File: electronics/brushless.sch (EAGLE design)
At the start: 70 parts, among them J1 USB_MINI-B_SMT, Q1 BUK7Y12-40E, Q2 BUK7Y12-40E, Q3 BUK7Y12-40E, Q4 BUK7Y12-40E, Q5 BUK7Y12-40E, Q6 BUK7Y12-40E, X1 JST-XH-10-PIN-LONG-PAD

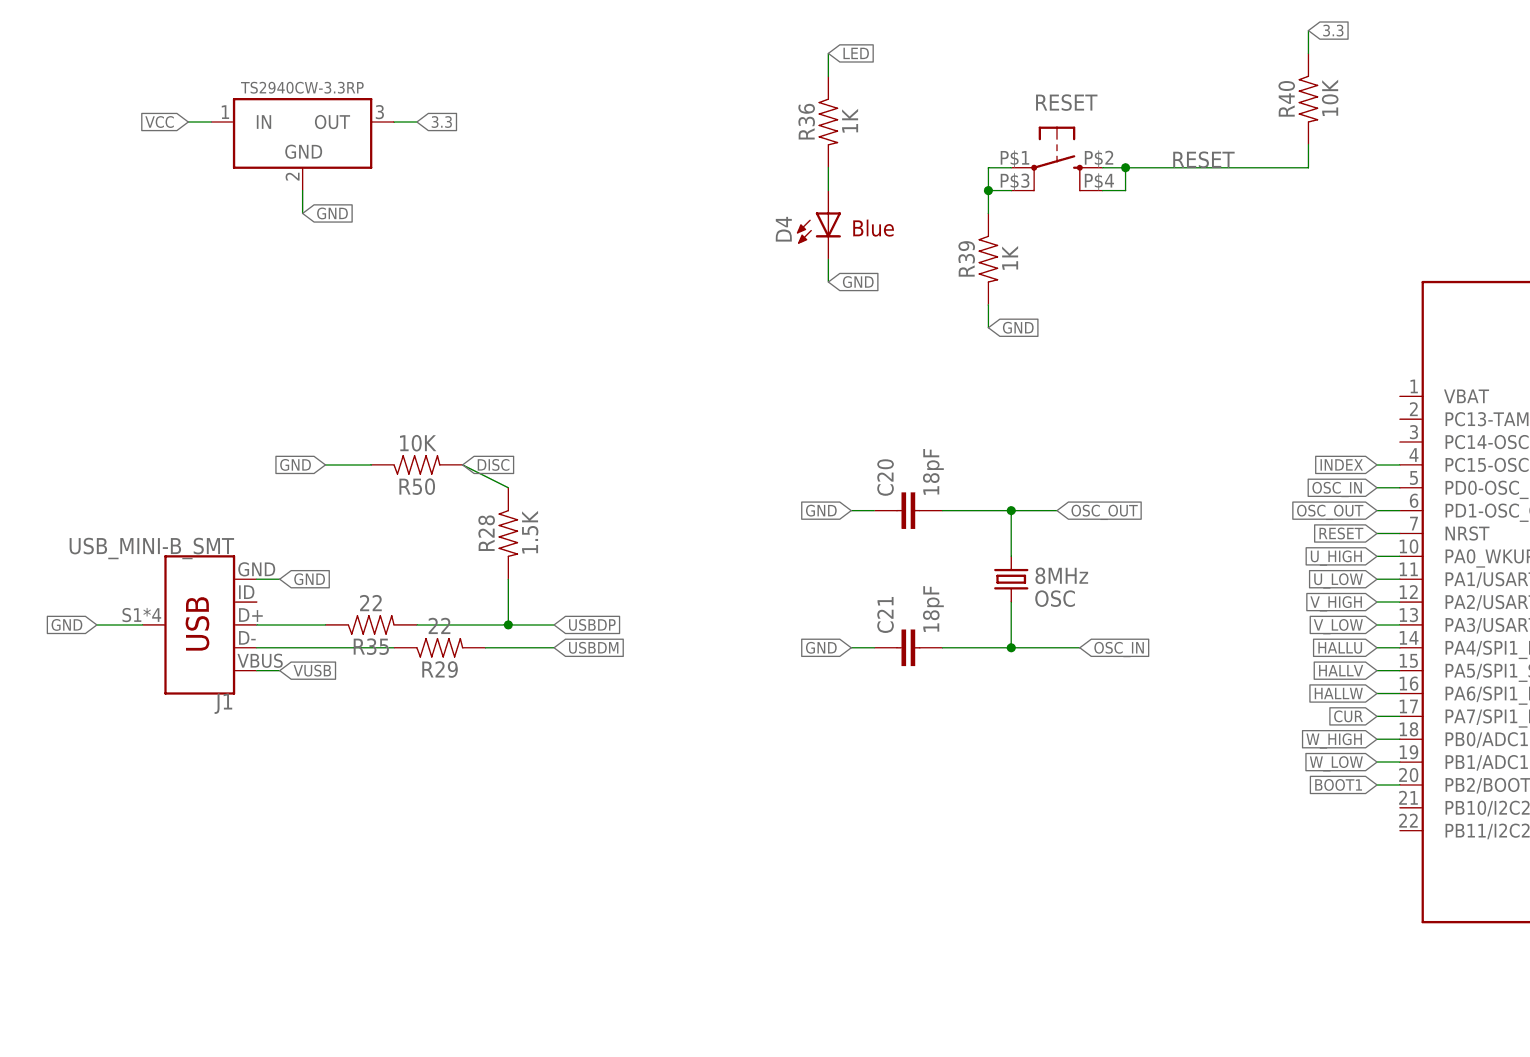
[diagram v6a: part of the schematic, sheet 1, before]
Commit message: Farnell refs & names
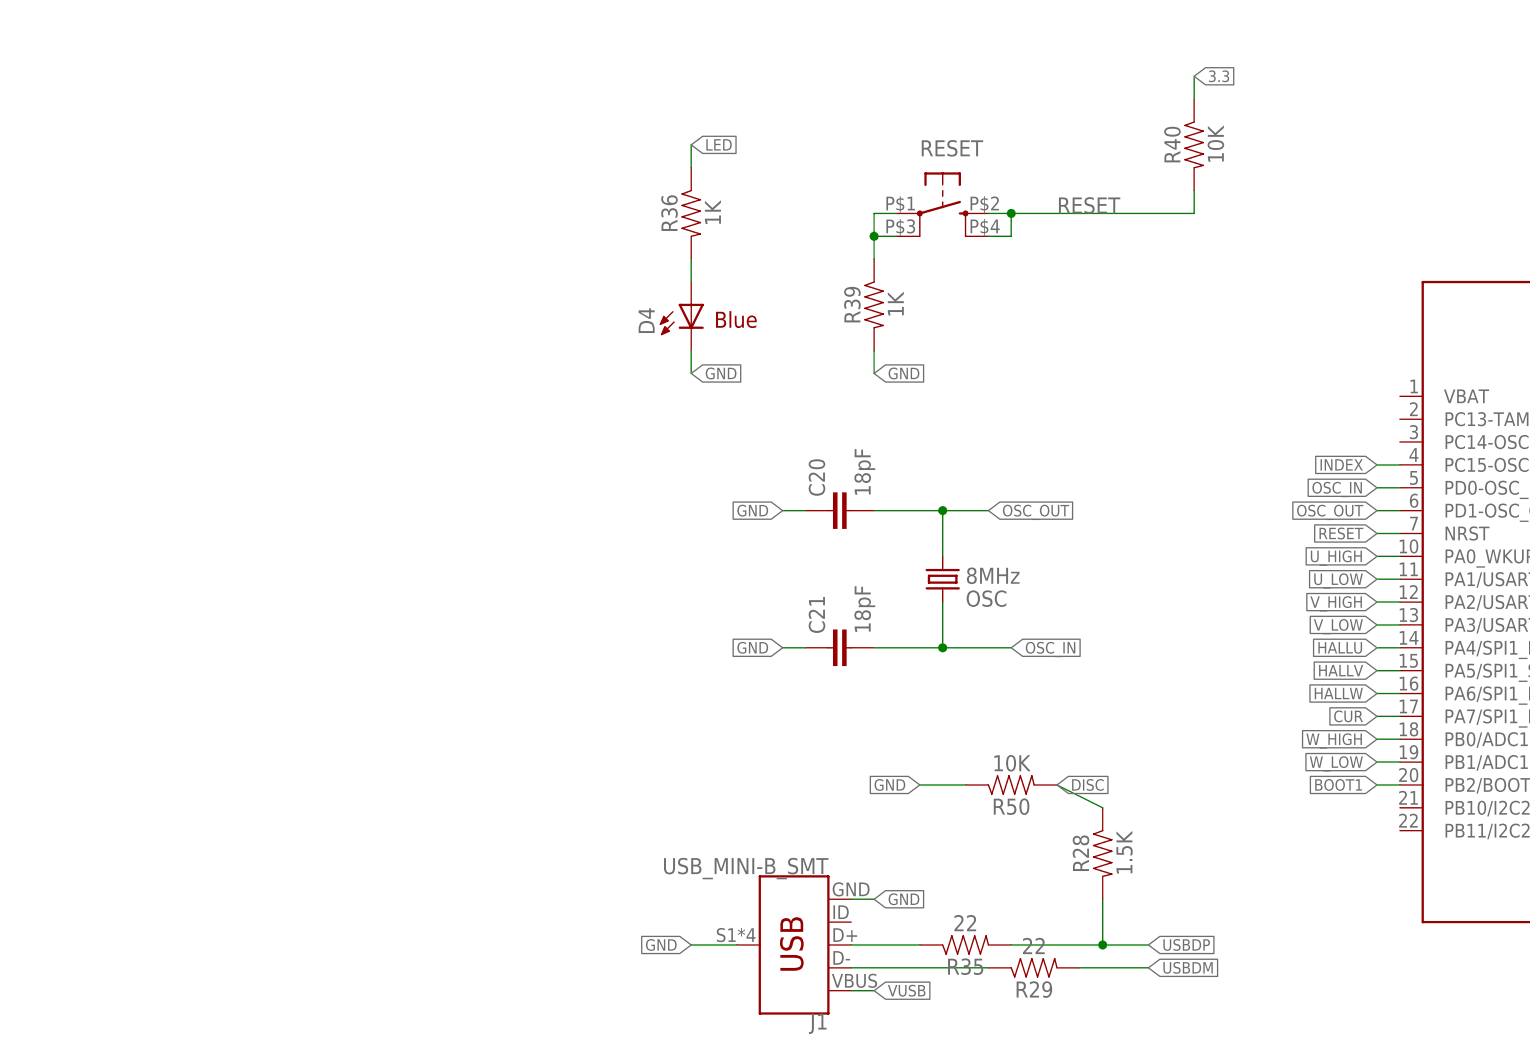
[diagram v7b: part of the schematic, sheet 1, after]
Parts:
- removed U$4: TS2940CW-3.3RP, rhoban:TS2940CW-3.3RP
- added REG1: TS2940CW-3.3RP, rhoban:TS2940CW-3.3RP
- BUT, RESET: FARNELL (none) -> 1437637
- C1, C2, C3: FARNELL (none) -> 2528772
- C12, C7: FARNELL (none) -> 2496946
- C17, C18: FARNELL (none) -> 721980
- C20, C21: FARNELL (none) -> 1414620
- C4: value 1nF -> 1000pF; FARNELL (none) -> 2496935
- D4: FARNELL (none) -> 1581233
- ENC1, R13, X1: FARNELL (none) -> -
- GND, V+: FARNELL (none) -> 1022248
- J1: FARNELL (none) -> 1753807
- LOGIC: FARNELL (none) -> 1022256
- OSC: FARNELL (none) -> 2467818
- OSC1: FARNELL (none) -> 1842013
- Q1, Q2, Q3, Q4, Q5, Q6: FARNELL (none) -> 2319916
- R1, R2, R3, R36, R39, R4, R49, R5, R6: FARNELL (none) -> 2446904
- R10, R11, R12, R14, R15, R16, R17, R18, R19, R23, R24, R25, R40, R48, R50, R7, R8, R9: FARNELL (none) -> 2447553
- R20: FARNELL (none) -> 2446939
- R21: FARNELL (none) -> 2446965
- R28: FARNELL (none) -> 2446909
- R29, R35: FARNELL (none) -> 2446926
- U$6: value (none) -> 100uF; FARNELL (none) -> 1144713
- U$7: FARNELL (none) -> 1329624
- renumbered U$1 to DRV1, U$2 to DRV2, U$3 to DRV3, U$5 to LOGIC
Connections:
- net 3.3: now also REG1.OUT; no longer U$4.OUT
- net GND: now also REG1.GND; no longer U$4.GND
- net VCC: now also REG1.IN; no longer U$4.IN
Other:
- note added: "CONNECTORS & POWER"
- note added: "STM32"
- note removed: "CONNECTORS"
- note removed: "MCU"
- moved on the sheet: C20, C21, D4, J1, OSC, R23, R24, R25, R28, R29, R35, R36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

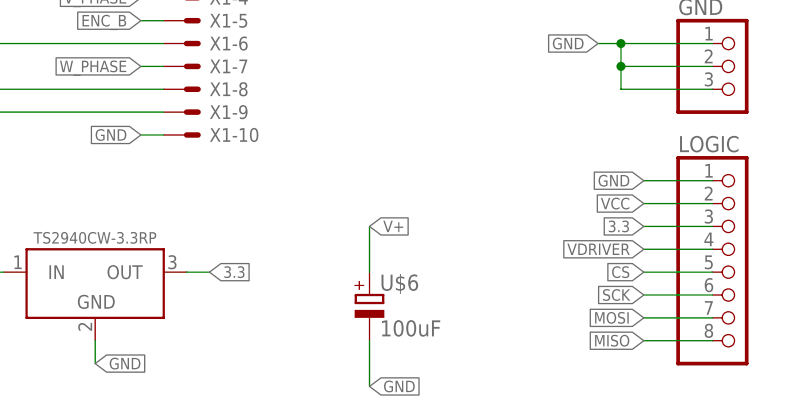
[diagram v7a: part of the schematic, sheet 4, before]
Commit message: bstop
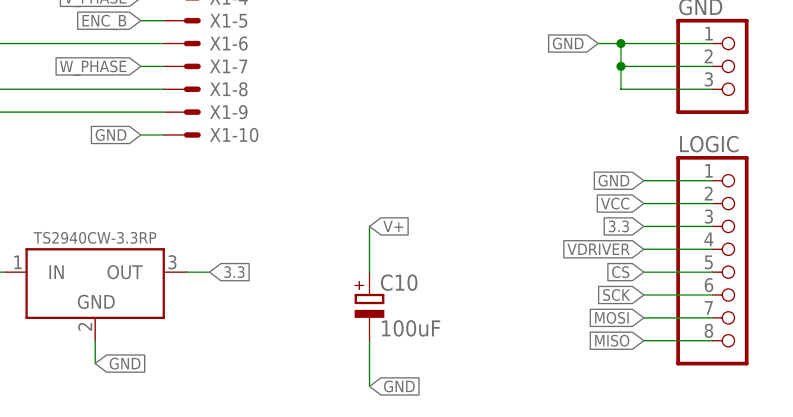
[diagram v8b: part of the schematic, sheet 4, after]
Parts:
- renumbered U$6 to C10, U$7 to SENSE
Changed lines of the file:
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@@
 <attribute name="FARNELL" value="1842013"/>
 </part>
-<part name="U$7" library="rhoban" deviceset="ACS712" device="">
+<part name="SENSE" library="rhoban" deviceset="ACS712" device="">
 <attribute name="FARNELL" value="1329624"/>
 </part>
@@
 <attribute name="FARNELL" value="7261403"/>
 </part>
-<part name="U$6" library="rhoban" deviceset="CPOL_EU" device="_3.5-8" value="100uF">
+<part name="C10" library="rhoban" deviceset="CPOL_EU" device="_3.5-8" value="100uF">
 <attribute name="FARNELL" value="1144713"/>
 </part>
@@
 <attribute name="FARNELL" x="109.22" y="20.32" size="1.778" layer="96" display="off"/>
 </instance>
-<instance part="U$7" gate="G$1" x="78.74" y="73.66">
+<instance part="SENSE" gate="G$1" x="78.74" y="73.66">
 <attribute name="FARNELL" x="78.74" y="73.66" size="1.778" layer="96" display="off"/>
 </instance>
@@
 </segment>
 <segment>
-<pinref part="U$7" gate="G$1" pin="GND"/>
+<pinref part="SENSE" gate="G$1" pin="GND"/>
 <wire x1="104.14" y1="76.2" x2="106.68" y2="76.2" width="0.1524" layer="91"/>
 <label x="106.68" y="76.2" size="1.27" layer="95" xref="yes"/>
@@
 <wire x1="71.12" y1="83.82" x2="71.12" y2="88.9" width="0.1524" layer="91"/>
 <label x="71.12" y="88.9" size="1.27" layer="95" rot="R90" xref="yes"/>
-<pinref part="U$7" gate="G$1" pin="IN-"/>
+<pinref part="SENSE" gate="G$1" pin="IN-"/>
 <wire x1="73.66" y1="78.74" x2="71.12" y2="83.82" width="0.1524" layer="91"/>
 </segment>
@@
 <pinref part="Q5" gate="G$1" pin="D"/>
 <wire x1="71.12" y1="60.96" x2="71.12" y2="78.74" width="0.1524" layer="91"/>
-<pinref part="U$7" gate="G$1" pin="IN+"/>
+<pinref part="SENSE" gate="G$1" pin="IN+"/>
 <wire x1="71.12" y1="78.74" x2="73.66" y2="83.82" width="0.1524" layer="91"/>
 </segment>
@@
 <net name="VCC" class="0">
 <segment>
-<pinref part="U$7" gate="G$1" pin="VCC"/>
+<pinref part="SENSE" gate="G$1" pin="VCC"/>
 <wire x1="104.14" y1="86.36" x2="106.68" y2="86.36" width="0.1524" layer="91"/>
 <label x="106.68" y="86.36" size="1.27" layer="95" rot="R90" xref="yes"/>
@@
 <net name="N$24" class="0">
 <segment>
-<pinref part="U$7" gate="G$1" pin="VIOUT"/>
+<pinref part="SENSE" gate="G$1" pin="VIOUT"/>
 <wire x1="104.14" y1="83.82" x2="106.68" y2="83.82" width="0.1524" layer="91"/>
 <pinref part="R20" gate="G$1" pin="1"/>
@@
 <net name="N$27" class="0">
 <segment>
-<pinref part="U$7" gate="G$1" pin="FILTER"/>
+<pinref part="SENSE" gate="G$1" pin="FILTER"/>
 <wire x1="104.14" y1="78.74" x2="114.3" y2="78.74" width="0.1524" layer="91"/>
 <pinref part="C4" gate="G$1" pin="1"/>
@@
 <attribute name="FARNELL" x="2.54" y="-25.4" size="1.778" layer="96" display="off"/>
 </instance>
-<instance part="U$6" gate="G$1" x="33.02" y="-30.48">
+<instance part="C10" gate="G$1" x="33.02" y="-30.48">
 <attribute name="FARNELL" x="33.02" y="-30.48" size="1.778" layer="96" display="off"/>
 </instance>
@@
 </segment>
 <segment>
-<pinref part="U$6" gate="G$1" pin="-"/>
+<pinref part="C10" gate="G$1" pin="-"/>
 <wire x1="33.02" y1="-33.02" x2="33.02" y2="-38.1" width="0.1524" layer="91"/>
 <label x="33.02" y="-38.1" size="1.27" layer="95" xref="yes"/>
@@
 </segment>
 <segment>
-<pinref part="U$6" gate="G$1" pin="+"/>
+<pinref part="C10" gate="G$1" pin="+"/>
 <wire x1="33.02" y1="-25.4" x2="33.02" y2="-20.32" width="0.1524" layer="91"/>
 <label x="33.02" y="-20.32" size="1.27" layer="95" xref="yes"/>
